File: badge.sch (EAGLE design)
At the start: 39 parts, among them SW1 MK12C02, SW2 MK12C02, U1 ESP8266, U2 AT25SF041-SOIC8, U3 LM317EMP-SOT223, U4 MCP73832T-2DCI/OT

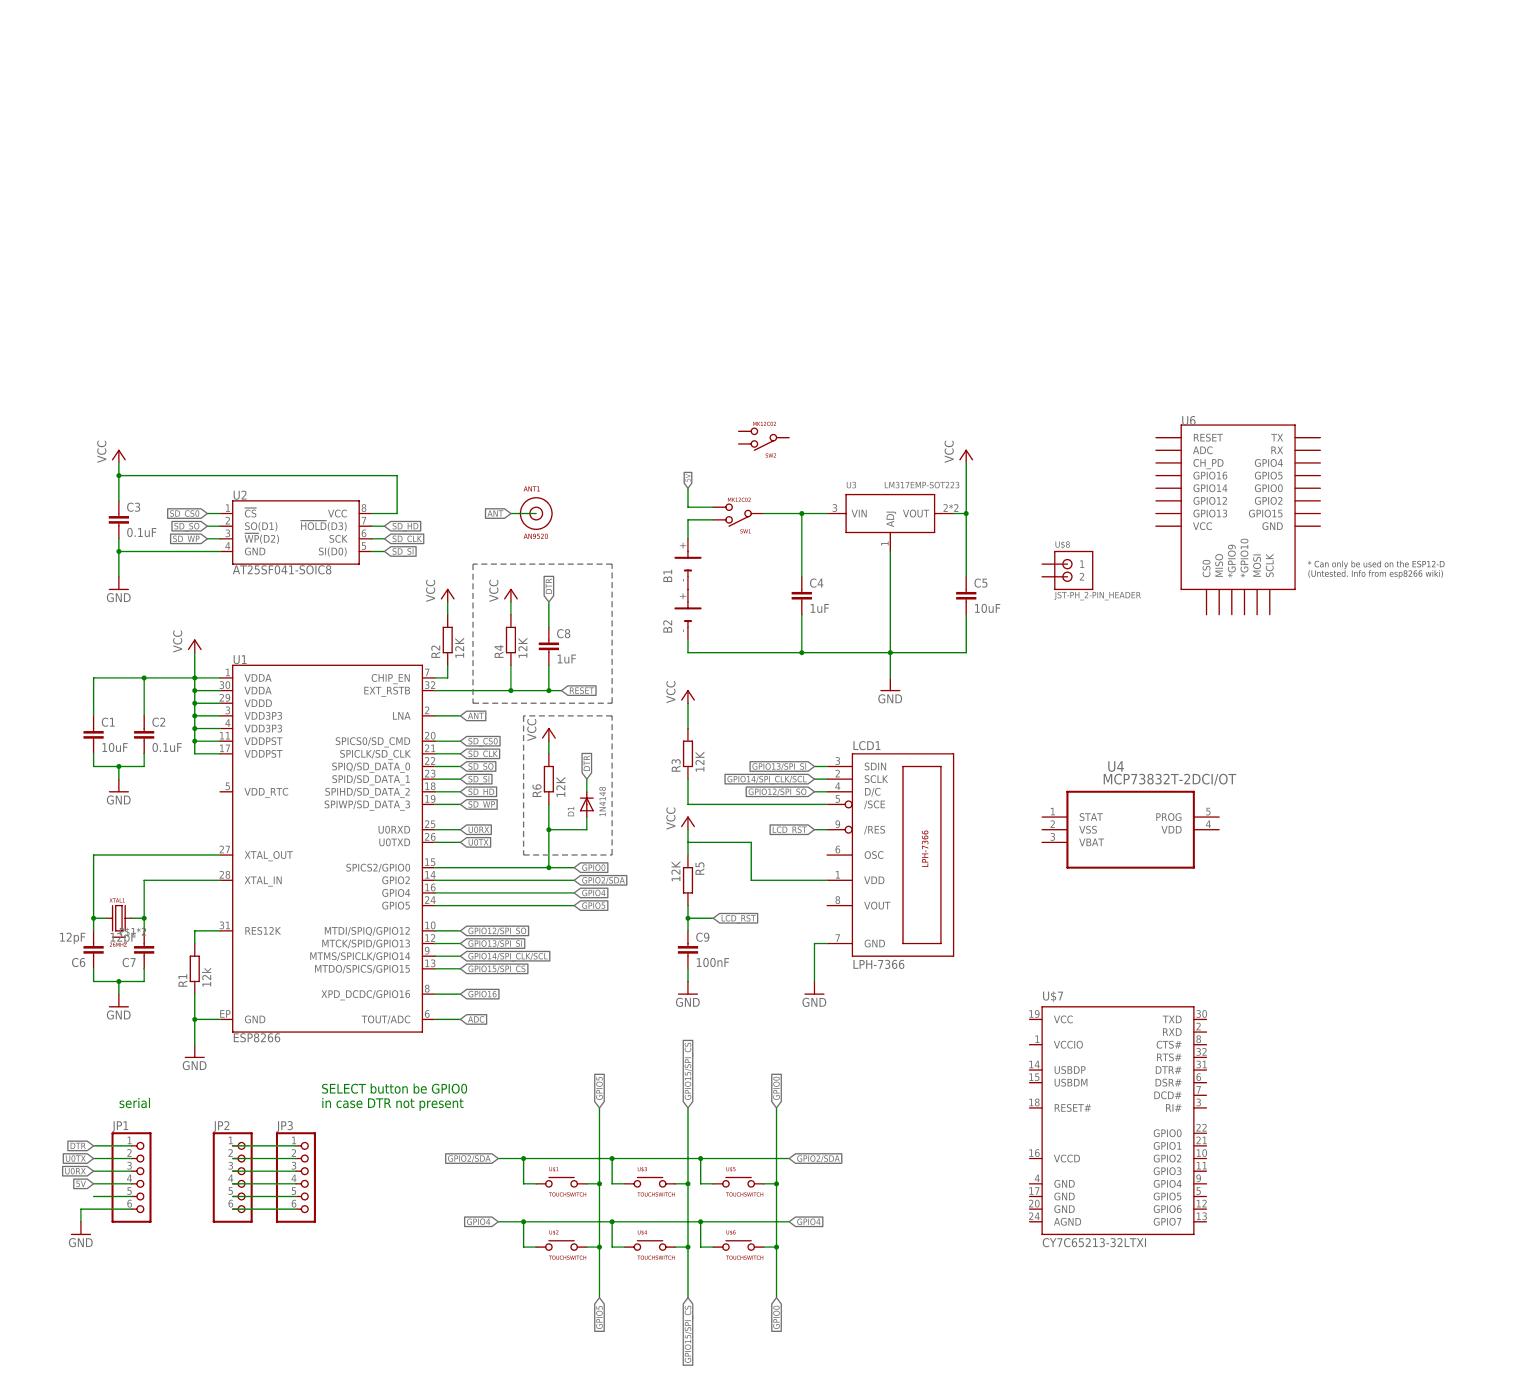
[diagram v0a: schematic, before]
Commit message: before the big change
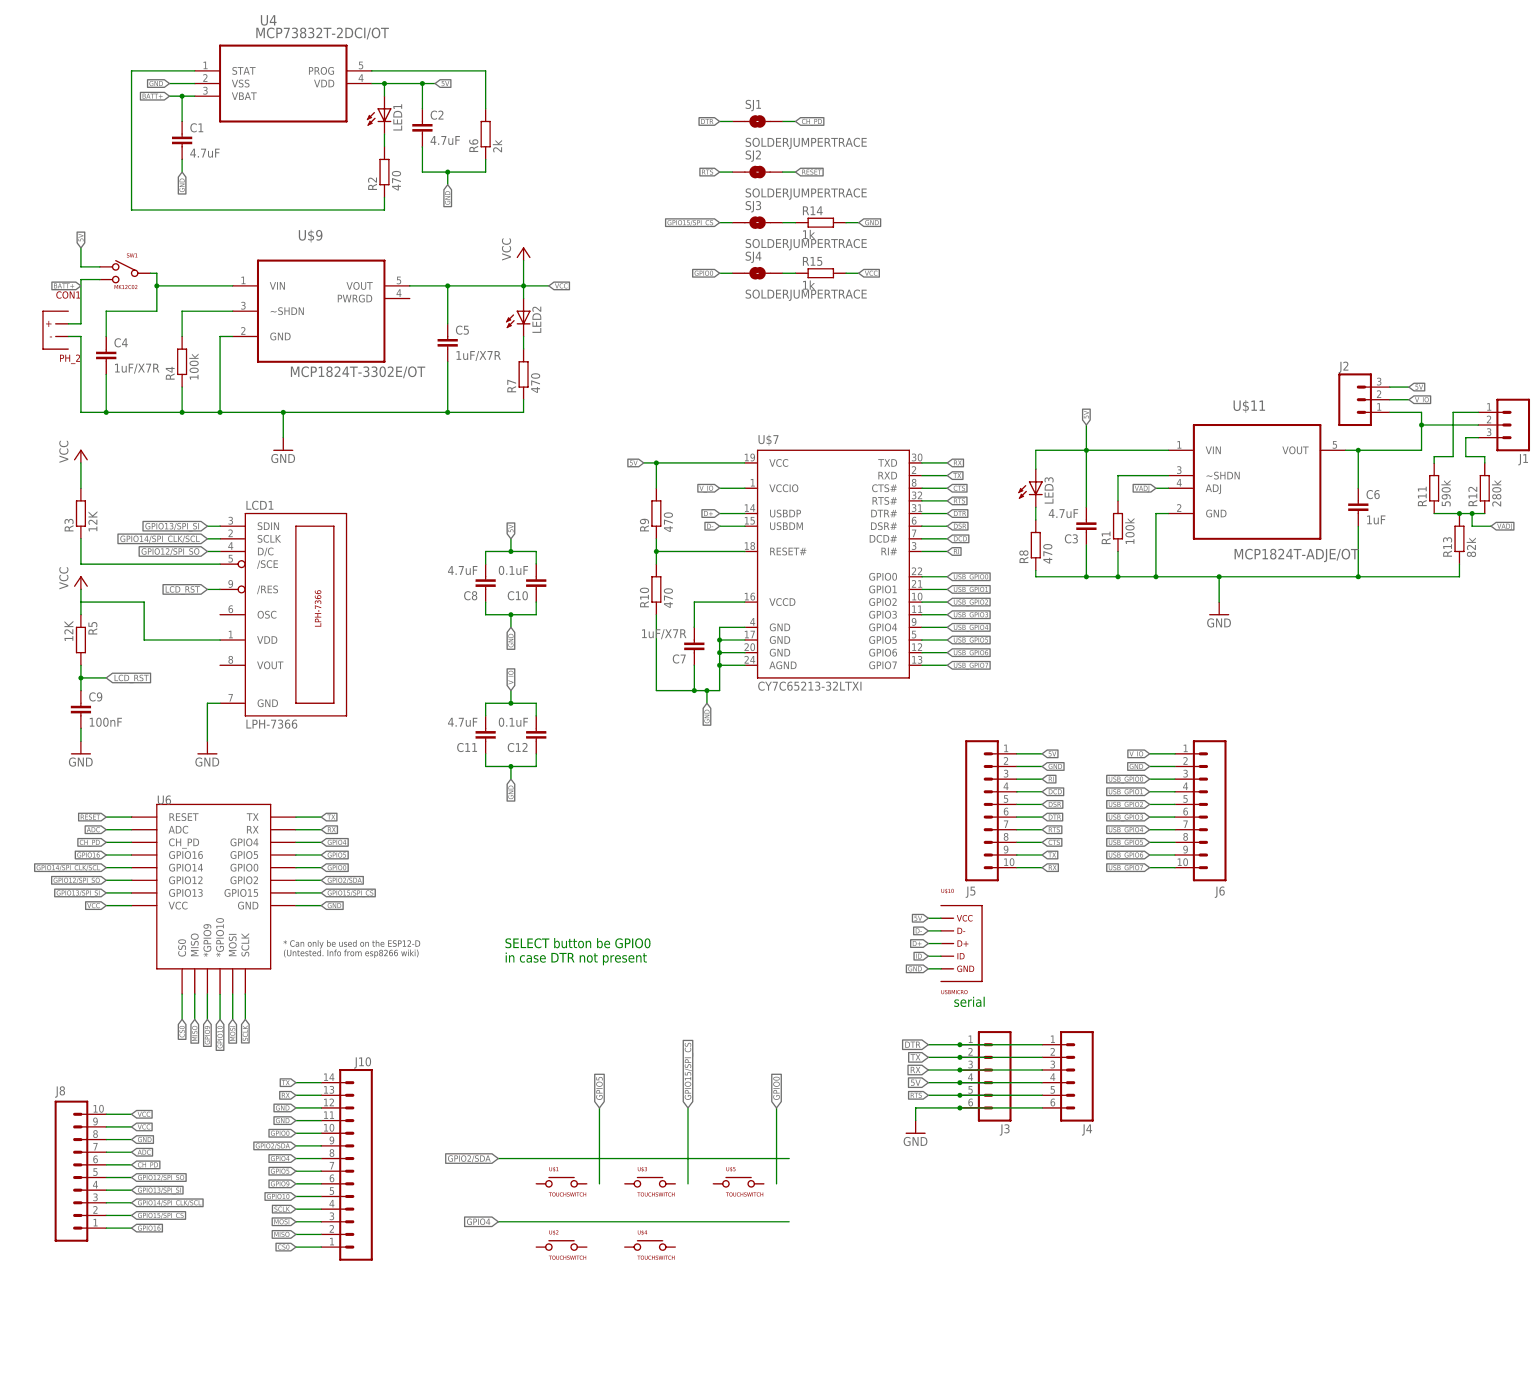
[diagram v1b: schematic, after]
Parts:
- removed ANT1: AN9520, badge:AN9520
- removed B1, B2: BATTERY, gm2:BATTERY
- removed D1: 1N4148, adafruit:DIODESOD-323F
- removed JP1, JP2, JP3: (no value), pinhead:PINHD-1X6
- removed SW2: MK12C02, badge:MK12C02
- removed U$6: TOUCHSWITCH, badge:TOUCHSWITCH
- removed U$8: JST-PH_2-PIN_HEADER, SRG:JST-PH_2-PIN_HEADER
- removed U1: ESP8266, SparkFun-RF:ESP8266
- removed U2: AT25SF041-SOIC8, SparkFun-RF:AT25SF041-SOIC8
- removed U3: LM317EMP-SOT223, Seeed-OPL-ic:PMIC-LDO-LM317EMP(SOT223)
- removed XTAL1: 26MHZ, badge:26MHZ
- added C10, C12: 0.1uF, resistor:C-EUC0603K
- added C11: 4.7uF, resistor:C-EUC0603K
- added CON1: PH_2, badge:PH_2
- added J1, J2: (no value), SparkFun-Connectors:M03PTH
- added J10: (no value), SparkFun-Connectors:M14
- added J3, J4: (no value), SparkFun-Connectors:M06SILK_FEMALE_PTH
- added J5, J6, J8: (no value), SparkFun-Connectors:M10SILK_FEMALE_PTH
- added LED1, LED2, LED3: (no value), led:LEDSML0805
- added R10, R7, R8, R9: 470, resistor:R-EU_R0603W
- added R11: 590k, resistor:R-EU_R0603W
- added R12: 280k, resistor:R-EU_R0603W
- added R13: 82k, resistor:R-EU_R0603W
- added R14, R15: 1k, resistor:R-EU_R0603W
- added SJ1, SJ2, SJ3, SJ4: SOLDERJUMPERTRACE, SparkFun-Retired:SOLDERJUMPERTRACE
- added U$10: USBMICRO, badge:USBMICRO
- added U$11: MCP1824T-ADJE/OT, Microchip_By_element14_Batch_1:MCP1824T-ADJE/OT
- added U$9: MCP1824T-3302E/OT, Microchip_By_element14_Batch_1:MCP1824T-3302E/OT
- C1: value 10uF -> 4.7uF
- C2, C3: value 0.1uF -> 4.7uF
- C4: value 1uF -> 1uF/X7R
- C5: value 10uF -> 1uF/X7R
- C6: value 12pF -> 1uF
- C7: value 12pF -> 1uF/X7R
- C8: value 1uF -> 4.7uF
- R1: value 12k -> 100k
- R2: value 12K -> 470
- R4: value 12K -> 100k
- R6: value 12K -> 2k
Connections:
- removed net ANT: ANT1.P$1, U1.LNA
- removed net N$13: JP2.5, JP3.5
- removed net N$14: JP2.6, JP3.6
- removed net N$15: JP1.5
- removed net N$2: R1.2, U1.RES12K
- removed net N$5: B1.+, SW1.P$2
- removed net N$8: C7.2, U1.XTAL_IN, XTAL1.P$2
- removed net SD_CLK: U1.SPICLK/SD_CLK, U2.SCK
- removed net SD_CS0: U1.SPICS0/SD_CMD, U2.!CS!
- removed net SD_HD: U1.SPIHD/SD_DATA_2, U2.!HOLD!(D3)
- removed net SD_SI: U1.SPID/SD_DATA_1, U2.SI(D0)
- removed net SD_SO: U1.SPIQ/SD_DATA_0, U2.SO(D1)
- removed net SD_WP: U1.SPIWP/SD_DATA_3, U2.!WP!(D2)
- removed net U0RX: JP1.3, U1.U0RXD
- removed net U0TX: JP1.2, U1.U0TXD
- new net BATT+: C1.1, CON1.P$1, SW1.P$3, U4.VBAT
- new net CH_PD: J8.6, SJ1.2, U6.CH_PD
- new net CS0: J10.1, U6.CS0
- new net CTS: J5.8, U$7.CTS#
- new net D+: U$10.P$D+, U$7.USBDP
- new net D-: U$10.P$D-, U$7.USBDM
- new net DCD: J5.4, U$7.DCD#
- new net DSR: J5.5, U$7.DSR#
- new net GPIO10: J10.5, U6.*GPIO10
- new net GPIO9: J10.6, U6.*GPIO9
- new net ID: U$10.P$ID
- new net MISO: J10.2, U6.MISO
- new net MOSI: J10.3, U6.MOSI
- new net N$16: J1.1, R11.2
- new net N$17: J1.3, R12.2
- new net N$18: R10.2, R9.1, U$7.RESET#
- new net N$19: C6.1, J1.2, J2.1, U$11.VOUT
- new net N$20: C7.2, U$7.VCCD
- new net N$28: R14.1, SJ3.2
- new net N$30: R15.1, SJ4.2
- new net RI: J5.3, U$7.RI#
- new net RTS: J3.5, J4.5, J5.7, SJ2.1, U$7.RTS#
- new net RX: J10.13, J3.3, J4.3, J5.10, U$7.TXD, U6.RX
- new net SCLK: J10.4, U6.SCLK
- new net TX: J10.14, J3.2, J4.2, J5.9, U$7.RXD, U6.TX
- new net USB_GPIO0: J6.3, U$7.GPIO0
- new net USB_GPIO1: J6.4, U$7.GPIO1
- new net USB_GPIO2: J6.5, U$7.GPIO2
- new net USB_GPIO3: J6.6, U$7.GPIO3
- new net USB_GPIO4: J6.7, U$7.GPIO4
- new net USB_GPIO5: J6.8, U$7.GPIO5
- new net USB_GPIO6: J6.9, U$7.GPIO6
- new net USB_GPIO7: J6.10, U$7.GPIO7
- new net VADJ: R11.1, R12.1, R13.2, U$11.ADJ
- new net V_IO: C11.2, C12.2, J2.2, J6.1, U$7.VCCIO
- net 5V: now also C10.2, C2.1, C3.2, C8.2, J2.3, J3.4, J4.4, J5.1, LED1.A, LED3.A, R9.2, SW1.P$2, U$10.P$VCC, U$11.VIN, U$7.VCC, U4.VDD; no longer JP1.4, SW1.P$3
- net ADC: now also J8.7, U6.ADC; no longer U1.TOUT/ADC
- net DTR: now also J3.1, J4.1, J5.6, SJ1.1, U$7.DTR#; no longer C8.1, D1.C, JP1.1
- net GND: now also C10.1, C11.1, C12.1, C3.1, C6.2, C8.1, CON1.P$2, J10.11, J10.12, J3.6, J4.6, J5.2, J6.2, J8.8, R10.1, R13.1, R14.2, R4.1, R6.1, R7.1, R8.1, U$10.P$GND, U$11.GND, U$7.AGND, U$7.GND@1, U$7.GND@2, U$7.GND@3, U$9.GND, U4.VSS, U6.GND; no longer B2.-, C3.2, C6.1, JP1.6, U1.GND, U2.GND, U3.ADJ
- net GPIO0: now also J10.10, SJ4.1, U6.GPIO0; no longer D1.A, R6.1, U$5.P$2, U$6.P$2, U1.SPICS2/GPIO0
- net GPIO12/SPI_SO: now also J8.5, U6.GPIO12; no longer U1.MTDI/SPIQ/GPIO12
- net GPIO13/SPI_SI: now also J8.4, U6.GPIO13; no longer U1.MTCK/SPID/GPIO13
- net GPIO14/SPI_CLK/SCL: now also J8.3, U6.GPIO14; no longer U1.MTMS/SPICLK/GPIO14
- net GPIO15/SPI_CS: now also J8.2, SJ3.1, U6.GPIO15; no longer U$3.P$2, U$4.P$2, U1.MTDO/SPICS/GPIO15
- net GPIO16: now also J8.1, U6.GPIO16; no longer U1.XPD_DCDC/GPIO16
- net GPIO2/SDA: now also J10.9, U6.GPIO2; no longer U$1.P$1, U$3.P$1, U$5.P$1, U1.GPIO2
- net GPIO4: now also J10.8, U6.GPIO4; no longer U$2.P$1, U$4.P$1, U$6.P$1, U1.GPIO4
- net GPIO5: now also J10.7, U6.GPIO5; no longer U$1.P$2, U$2.P$2, U1.GPIO5
- net N$1: now also U$9.VIN; no longer U3.VIN
- net N$10: now also R2.1, U4.STAT; no longer JP2.2, JP3.2
- net N$11: now also R1.2, U$11.~SHDN; no longer JP2.3, JP3.3
- net N$12: now also LED3.C, R8.2; no longer JP2.4, JP3.4
- net N$4: now also R4.2, U$9.~SHDN; no longer R2.1, U1.CHIP_EN
- net N$6: now also R6.2, U4.PROG; no longer C6.2, U1.XTAL_OUT, XTAL1.P$1
- net N$7: now also LED2.C, R7.2; no longer JP2.1, JP3.1
- net N$9: now also LED1.C, R2.2; no longer B1.-, B2.+
- net RESET: now also SJ2.2, U6.RESET; no longer C8.2, R4.1, U1.EXT_RSTB
- net VCC: now also J8.10, J8.9, LED2.A, R15.2, U$9.VOUT, U6.VCC; no longer C1.1, C2.1, C3.1, R2.2, R4.2, R6.2, U1.VDD3P3@3, U1.VDD3P3@4, U1.VDDA@1, U1.VDDA@30, U1.VDDD, U1.VDDPST@11, U1.VDDPST@17, U2.VCC, U3.VOUT
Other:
- moved on the sheet: C1, C2, C3, C4, C5, C6, C7, C8, C9, LCD1, R1, R2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
